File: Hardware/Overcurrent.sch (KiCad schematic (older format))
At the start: 20 parts, among them Q3 BSS138, SW2 SW_Push, U11 LM285D-1.2, U12 74AHCT1G04, U13 74LVC1G08, U14 TC75S57F, U15 74LVC2G02, U16 TC4452

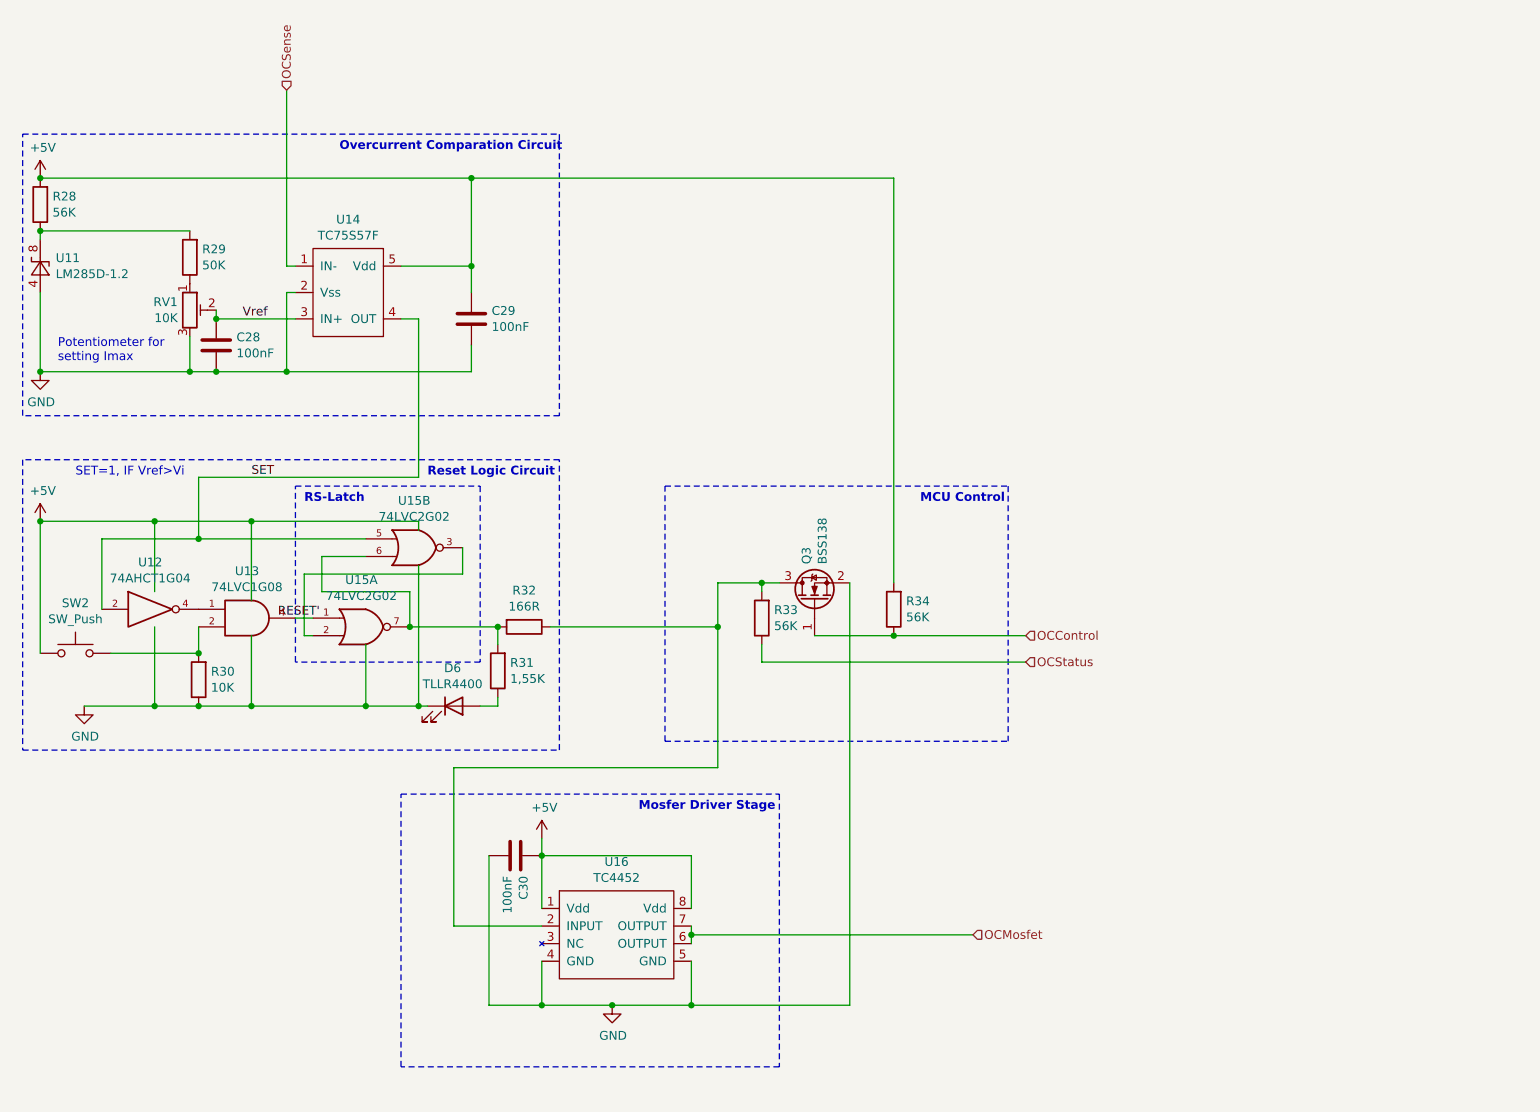
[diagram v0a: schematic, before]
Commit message: changed the OC logic
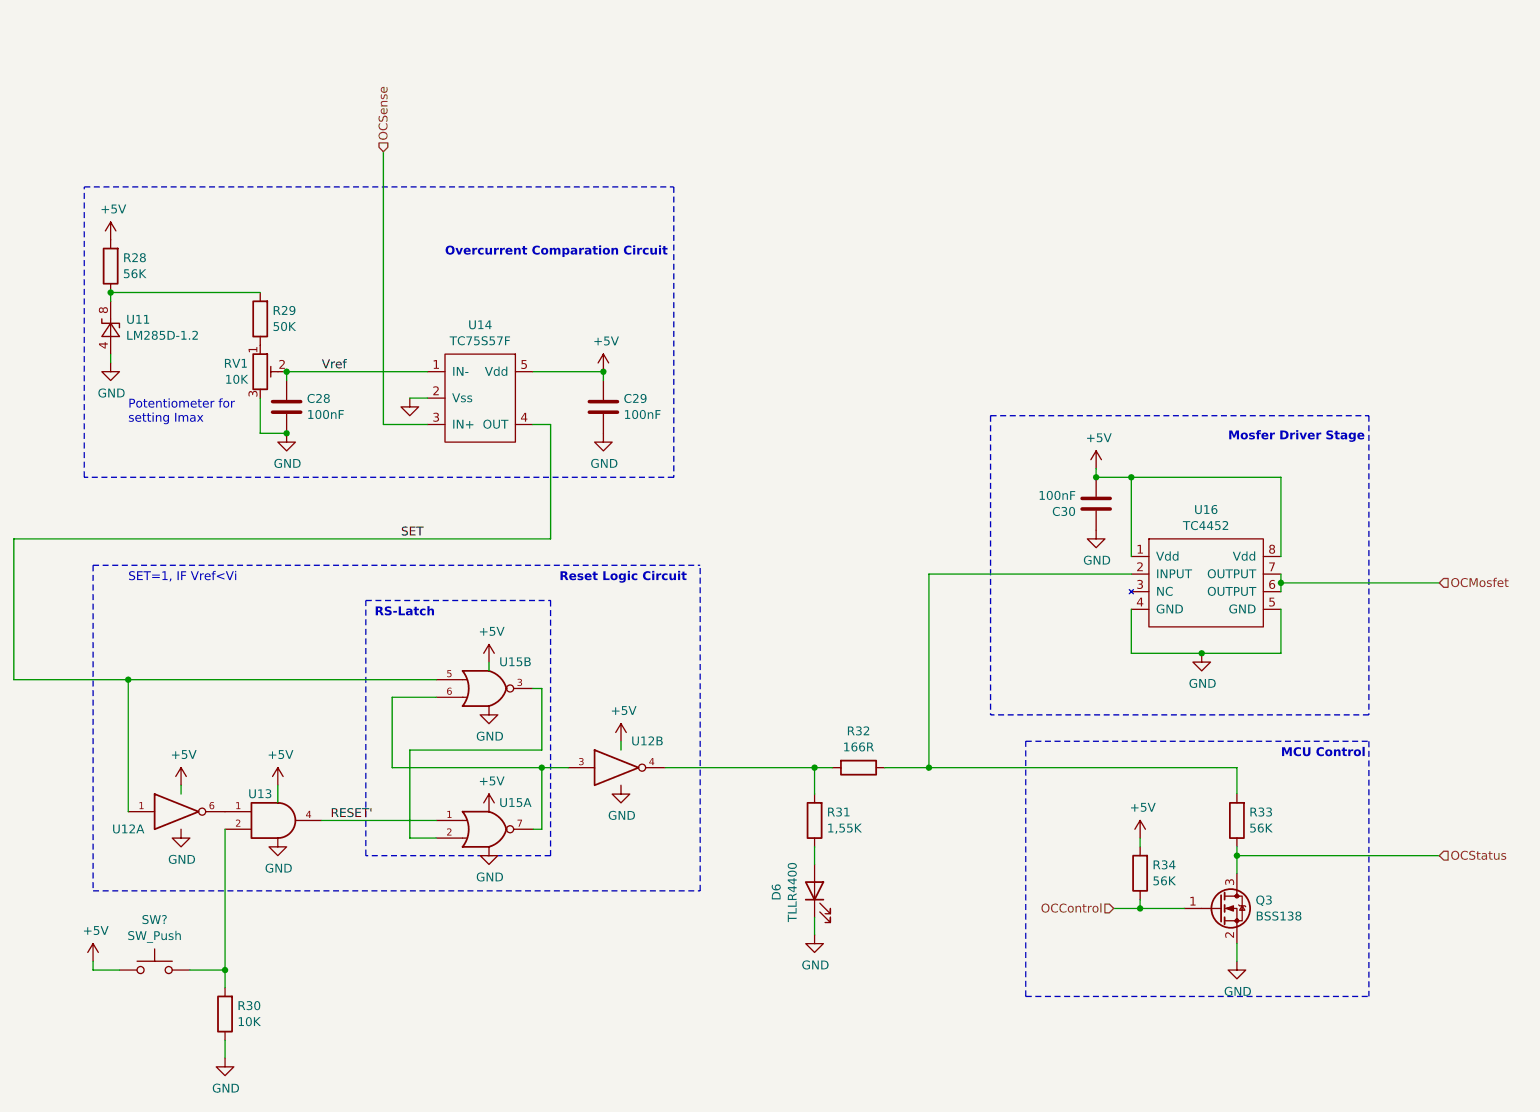
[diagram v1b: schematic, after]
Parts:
- removed SW2: SW_Push, symbol Switch:SW_Push
- removed U12: 74AHCT1G04, symbol 74xGxx:74AHCT1G04
- added SW?: SW_Push, symbol Switch:SW_Push
- added U12: 74LVC2G04, symbol 74xGxx:74LVC2G04
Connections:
- net +5V: now also C30.1, SW?.1, U12.5 (VCC), U12.5 (VCC); no longer C30.2
- net GND: now also C30.2, U12.2 (GND), U12.2 (GND); no longer C30.1
- net OCSense: now also U14.3 (IN+); no longer U14.1 (IN-)
- net OCStatus: now also Q3.3 (D)
- net RESET': now also U13.4, U15.1
- net SET: now also U12.1
- net Vref: now also U14.1 (IN-); no longer U14.3 (IN+)
- net at R32.1, R33.2, U16.2 (INPUT): no longer Q3.3 (D)
- net at U13.1: now also U12.6
- net at R30.2, U13.2: now also SW?.2
- net at R31.2, R32.2: now also U12.4; no longer U15.6, U15.7
- new net: U12.3, U15.6, U15.7
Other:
- note added: "SET=1, IF Vref<Vi"
- note removed: "SET=1, IF Vref>Vi"
- moved on the sheet: C28, C29, C30, D6, Q3, R28, R29, R30, R31, R32, R33, R34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
